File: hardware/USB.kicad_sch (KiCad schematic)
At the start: 24 parts, among them J3 USB_A, P4 USB_C_Plug_USB2.0, Q1 DMG3415U-7, SW1 ON, SW4 SWITCH, U1 USB3740B-AI9

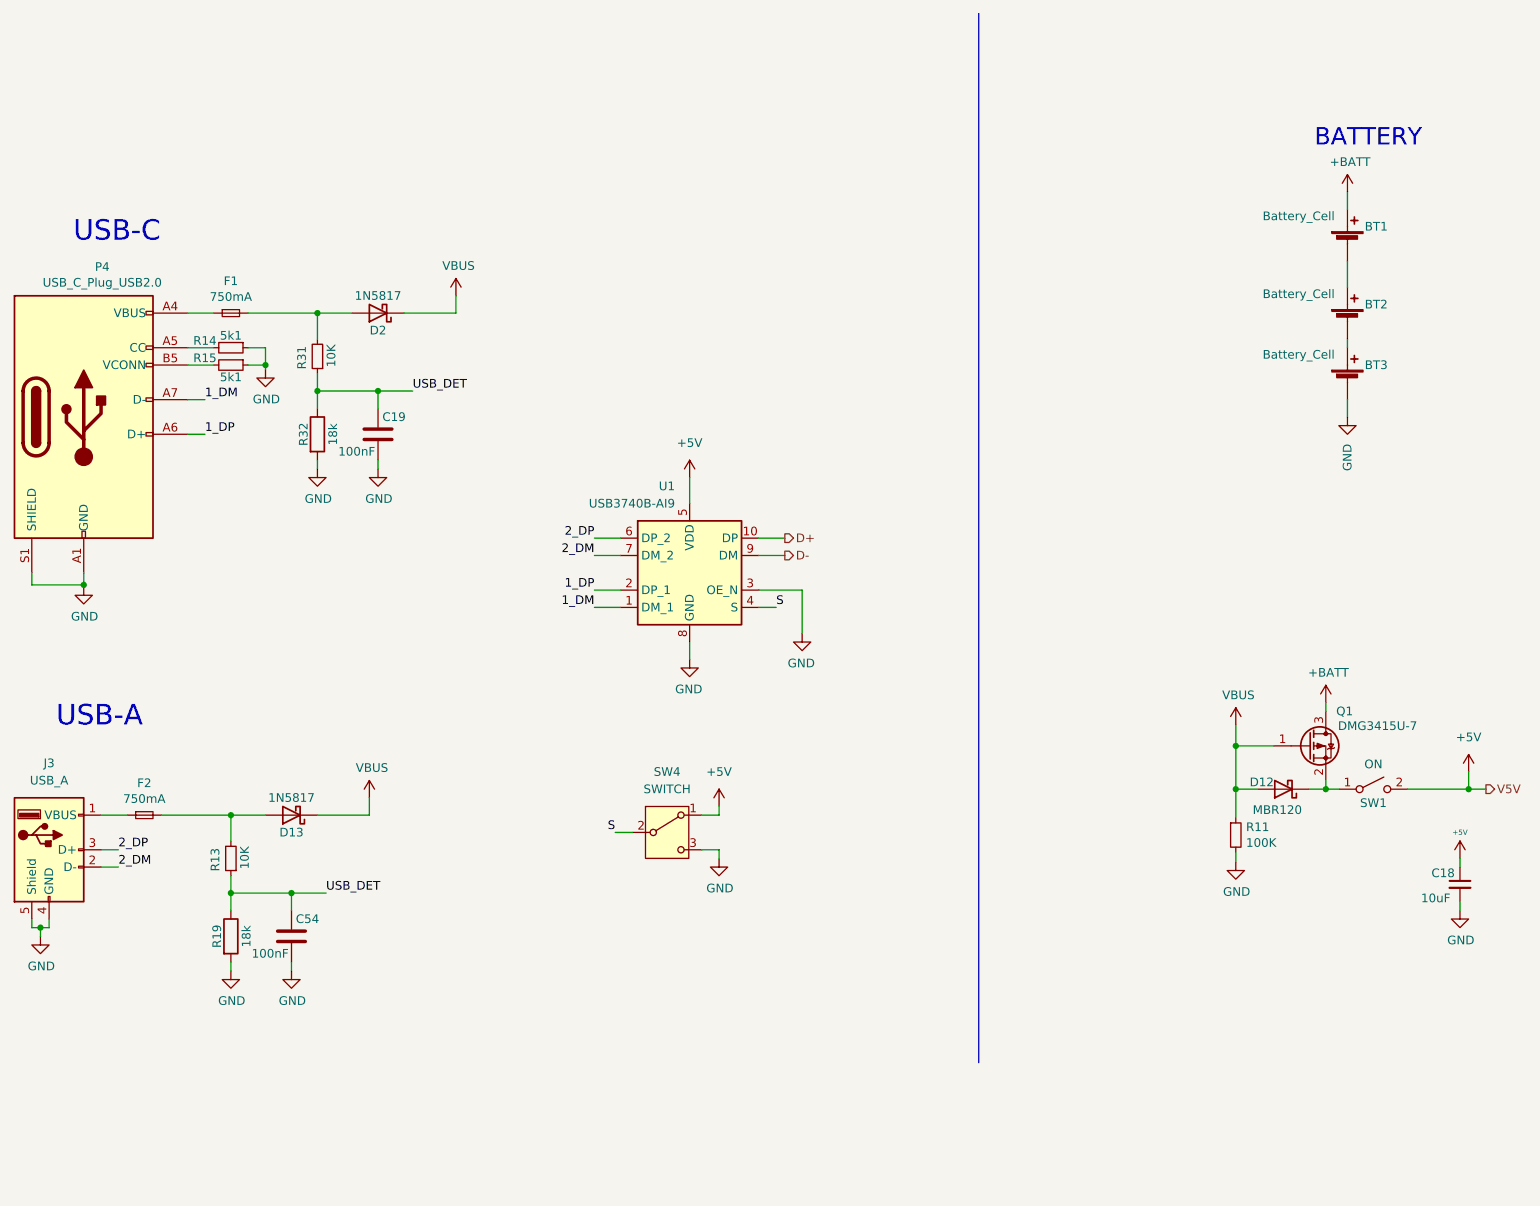
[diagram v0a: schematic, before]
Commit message: feat(Hw):Update_Schematic
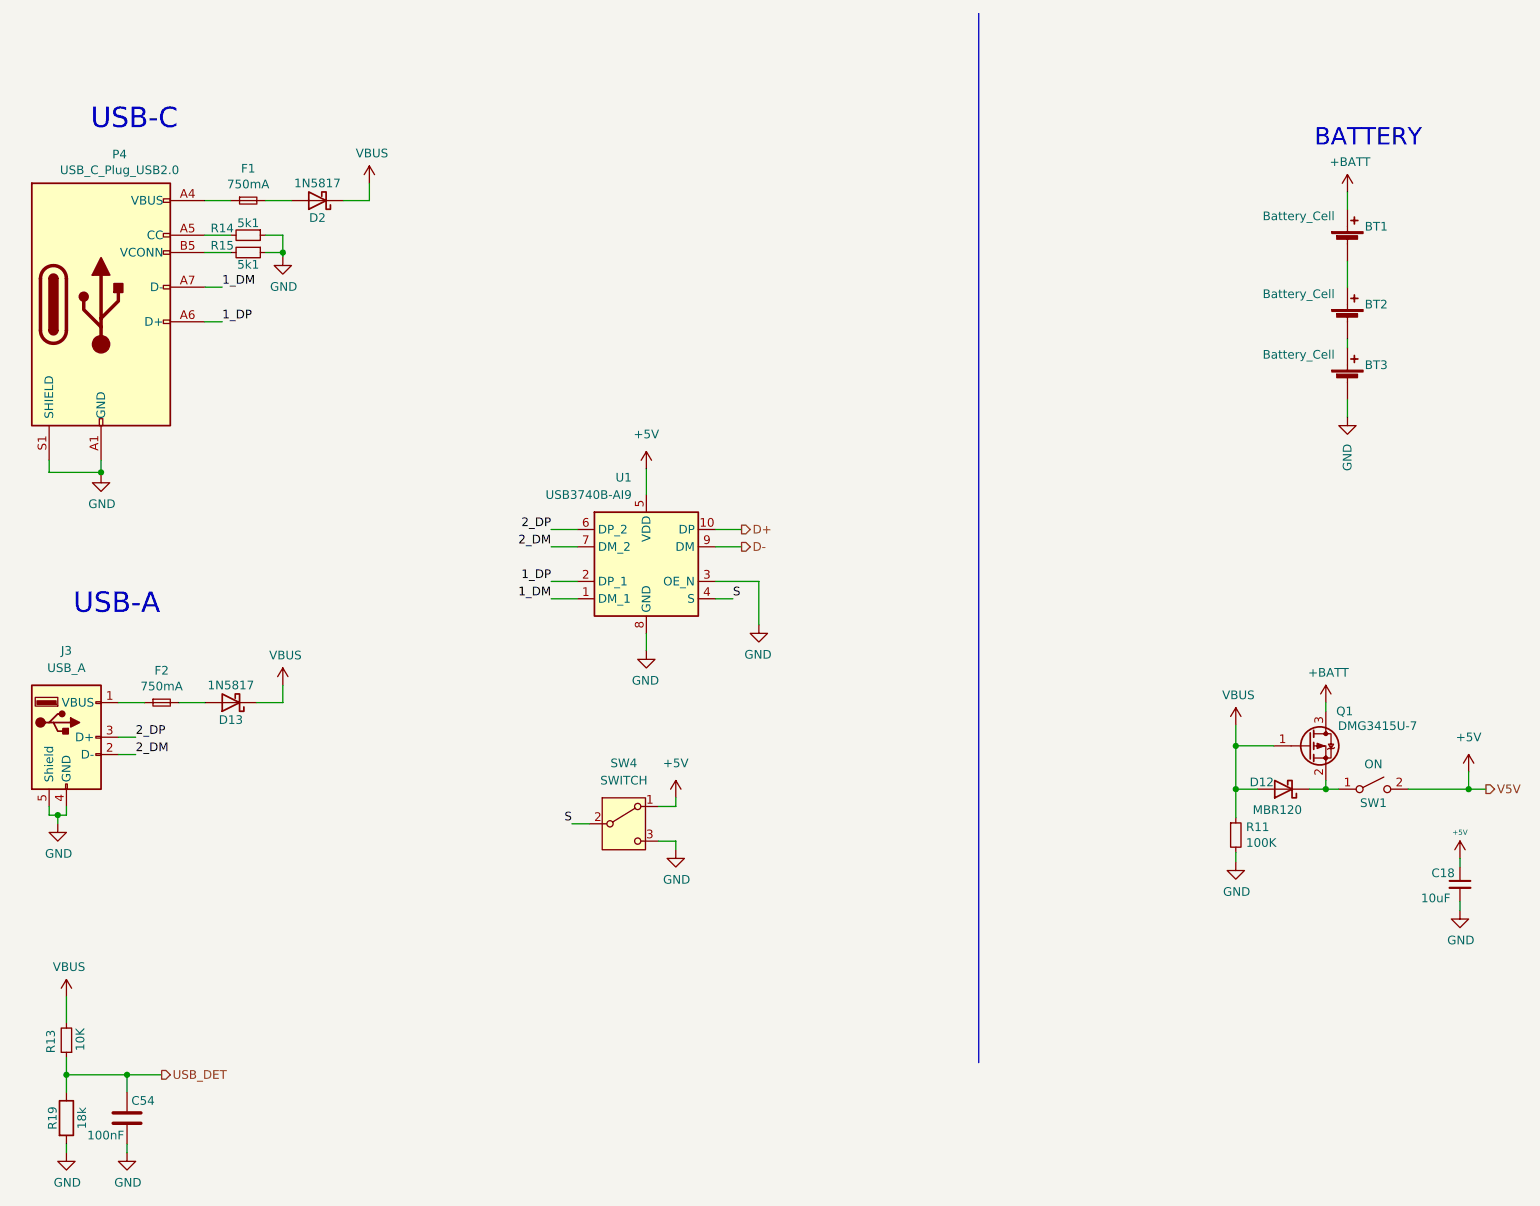
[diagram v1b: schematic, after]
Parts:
- removed C19: 100nF, Capacitor_SMD:C_0402_1005Metric, symbol Device:C
- removed R31: 10K, Resistor_SMD:R_0402_1005Metric, symbol Device:R_Small
- removed R32: 18k, Resistor_SMD:R_0402_1005Metric, symbol Device:R
- BT1, BT2, BT3: #LCSC C5290189 -> (none)
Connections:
- net VBUS: now also R13.2
- net at D13.2 (A), F2.2: no longer R13.2
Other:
- moved on the sheet: C54, D13, D2, F1, F2, J3, P4, R13, R14, R15, R19, SW4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
